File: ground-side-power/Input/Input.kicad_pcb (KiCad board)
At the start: 2 copper layers, 100.3 x 130 mm, 41 parts, among them J1 Battery Terminals, J2 Battery Terminals, J26 Conn_01x02_Female, J3 Battery Terminals, J4 Battery Terminals, J5 455860005, J6 455860005, J7 ATX-24, J8 Conn_01x03_Female, J9 Conn_01x03_Female, K1 AZ2150-1A-12DEF, M1 Fan_PC_Chassis, SW1 GRB234A2NABA1, U1 INA180, U2 INA180

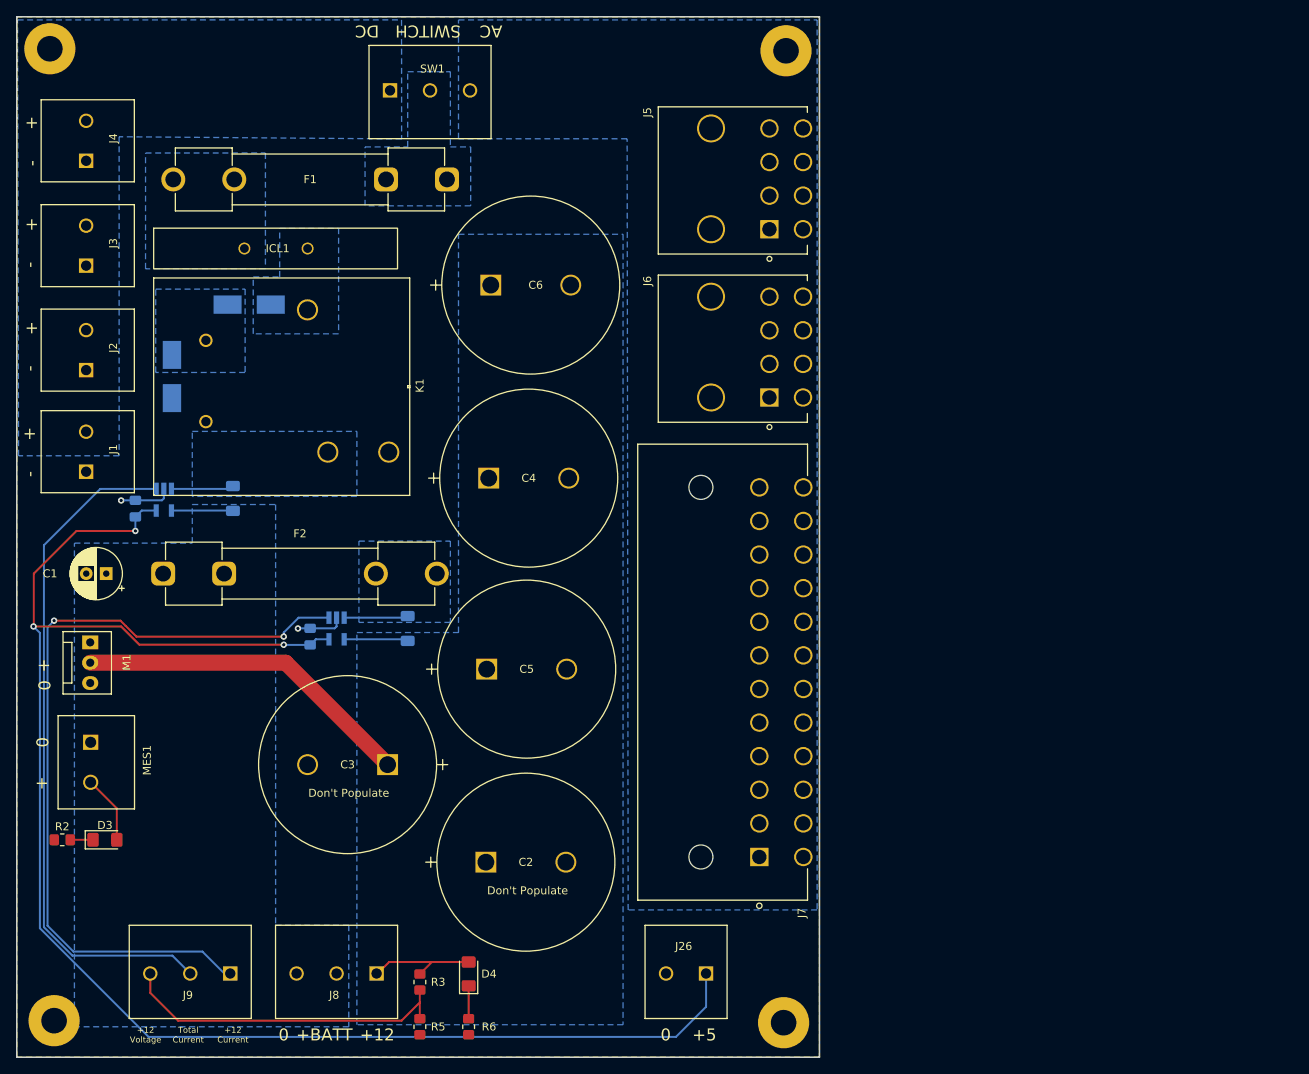
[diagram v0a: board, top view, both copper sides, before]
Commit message: Resolved Final Issues
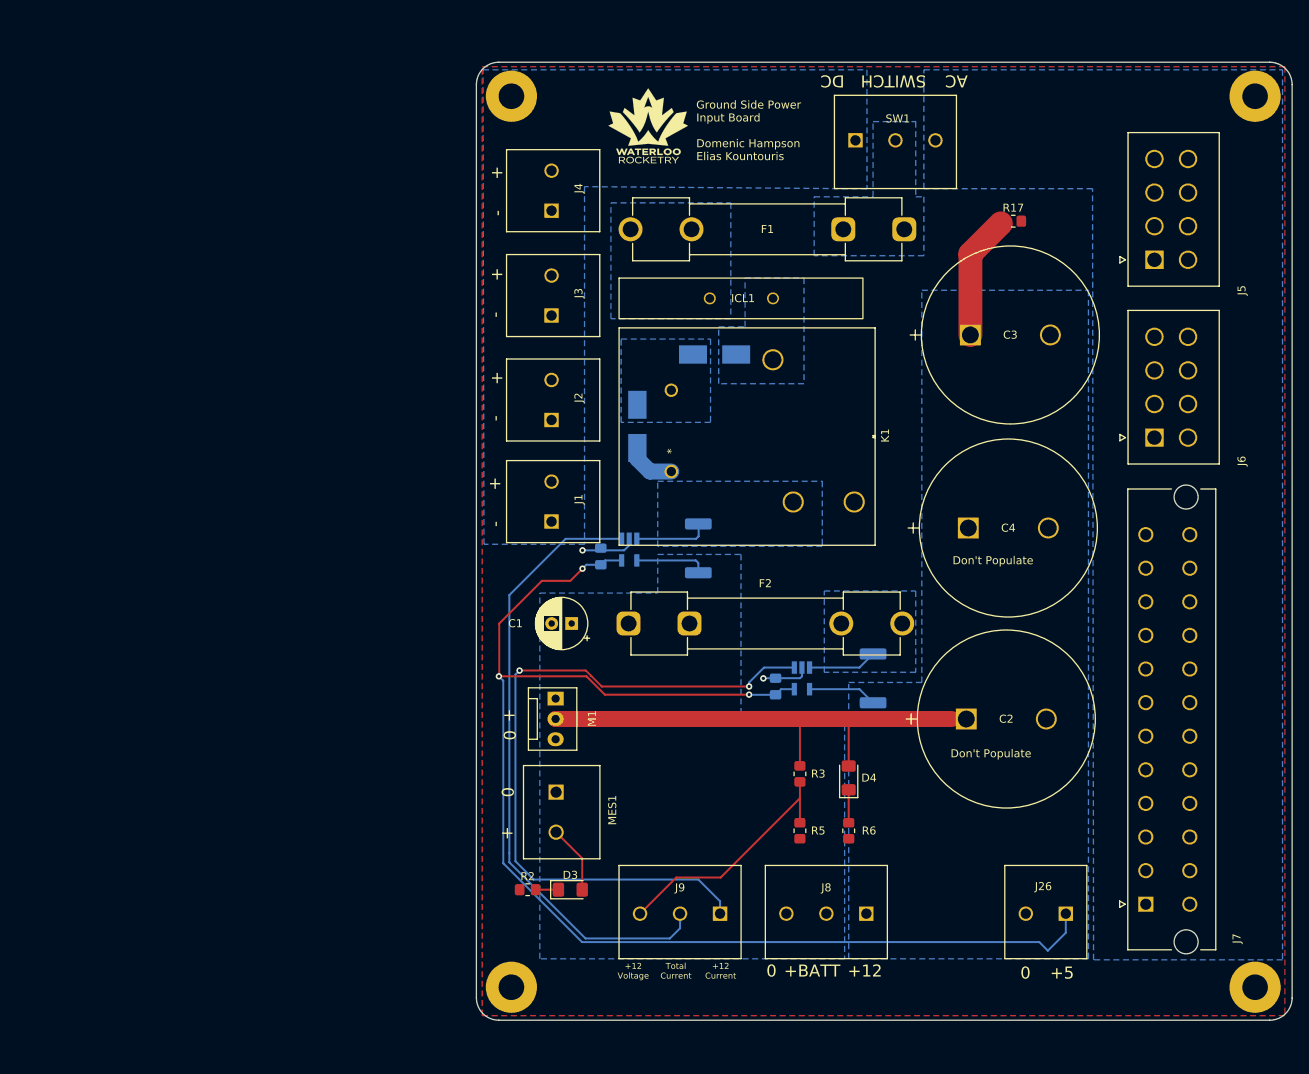
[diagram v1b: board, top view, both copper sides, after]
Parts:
- removed C5, C6: 22mF, GSP:LLS1C223MELZ
- added G***: LOGO, rlcs:rocketry_logo_small, F.Cu at (119.5, 46.1)
- added R17: 10k, Resistor_SMD:R_0805_2012Metric_Pad1.20x1.40mm_HandSolder, F.Cu at (165.1, 58.1)
- J5, J6: value 455860005 -> 874270842; footprint GSP:MOLEX_455860005 -> GSP:MOLEX_874270842
- J7: footprint GSP:MOLEX_15246240 -> GSP:MOLEX_442060001
- R1, R4: value 0.0016 -> 0.0015; footprint Resistor_SMD:R_1206_3216Metric_Pad1.30x1.75mm_HandSolder -> Resistor_SMD:R_2512_6332Metric_Pad1.40x3.35mm_HandSolder
- moved C3 90.5 mm to (159.7, 72.3), turned to 0 degrees
- moved C2 62.7 mm to (159.2, 120.3)
- moved J9 61.7 mm to (128.5, 144.6)
- moved J8 61.7 mm to (146.7, 144.6)
- moved C4 60.3 mm to (159.5, 96.4)
- moved ? 59.1 mm to (195.3, 153.8)
- moved ? 58.9 mm to (195.3, 42.4)
- moved M1 58.6 mm to (107.9, 117.7)
- moved ICL1 58.5 mm to (131.1, 67.7)
- moved C1 58.5 mm to (109.9, 108.3)
- moved J1 58.5 mm to (107.4, 95.6)
- moved J2 58.5 mm to (107.4, 82.9)
- moved J3 58.5 mm to (107.4, 69.8)
- moved J4 58.5 mm to (107.4, 56.7)
- moved C7 58.5 mm to (135.4, 116.2)
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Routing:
- net +5V: track 197.1 -> 165.1 mm
- net +12V: track 64.7 -> 85.6 mm
- net /12_VOLTAGE: track 42.1 -> 31.1 mm
- net /12V_OUT: track 100.2 -> 89.7 mm
- net /TOTAL_OUT: track 85.4 -> 78.0 mm
- net GND: track 12.7 -> 19.2 mm
- net /Sys_Sense+: track 7.72 -> 9.41 mm
- net +BATT: track 16.4 -> 17.6 mm
- net /12V_Sense+: track 8.02 -> 8.64 mm
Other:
- board size 100.3 x 130 mm -> 102 x 119.7 mm
- board text added: "Ground Side Power Input Board Domenic Hampson Elias Kountouris"
